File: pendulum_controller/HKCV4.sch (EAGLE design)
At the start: 56 parts, among them Q1 TPH, Q2 TPH, Q3 TPH, Q4 TPH, Q5 TPH, Q6 TPH, U1 LTC2851MPDDPBF

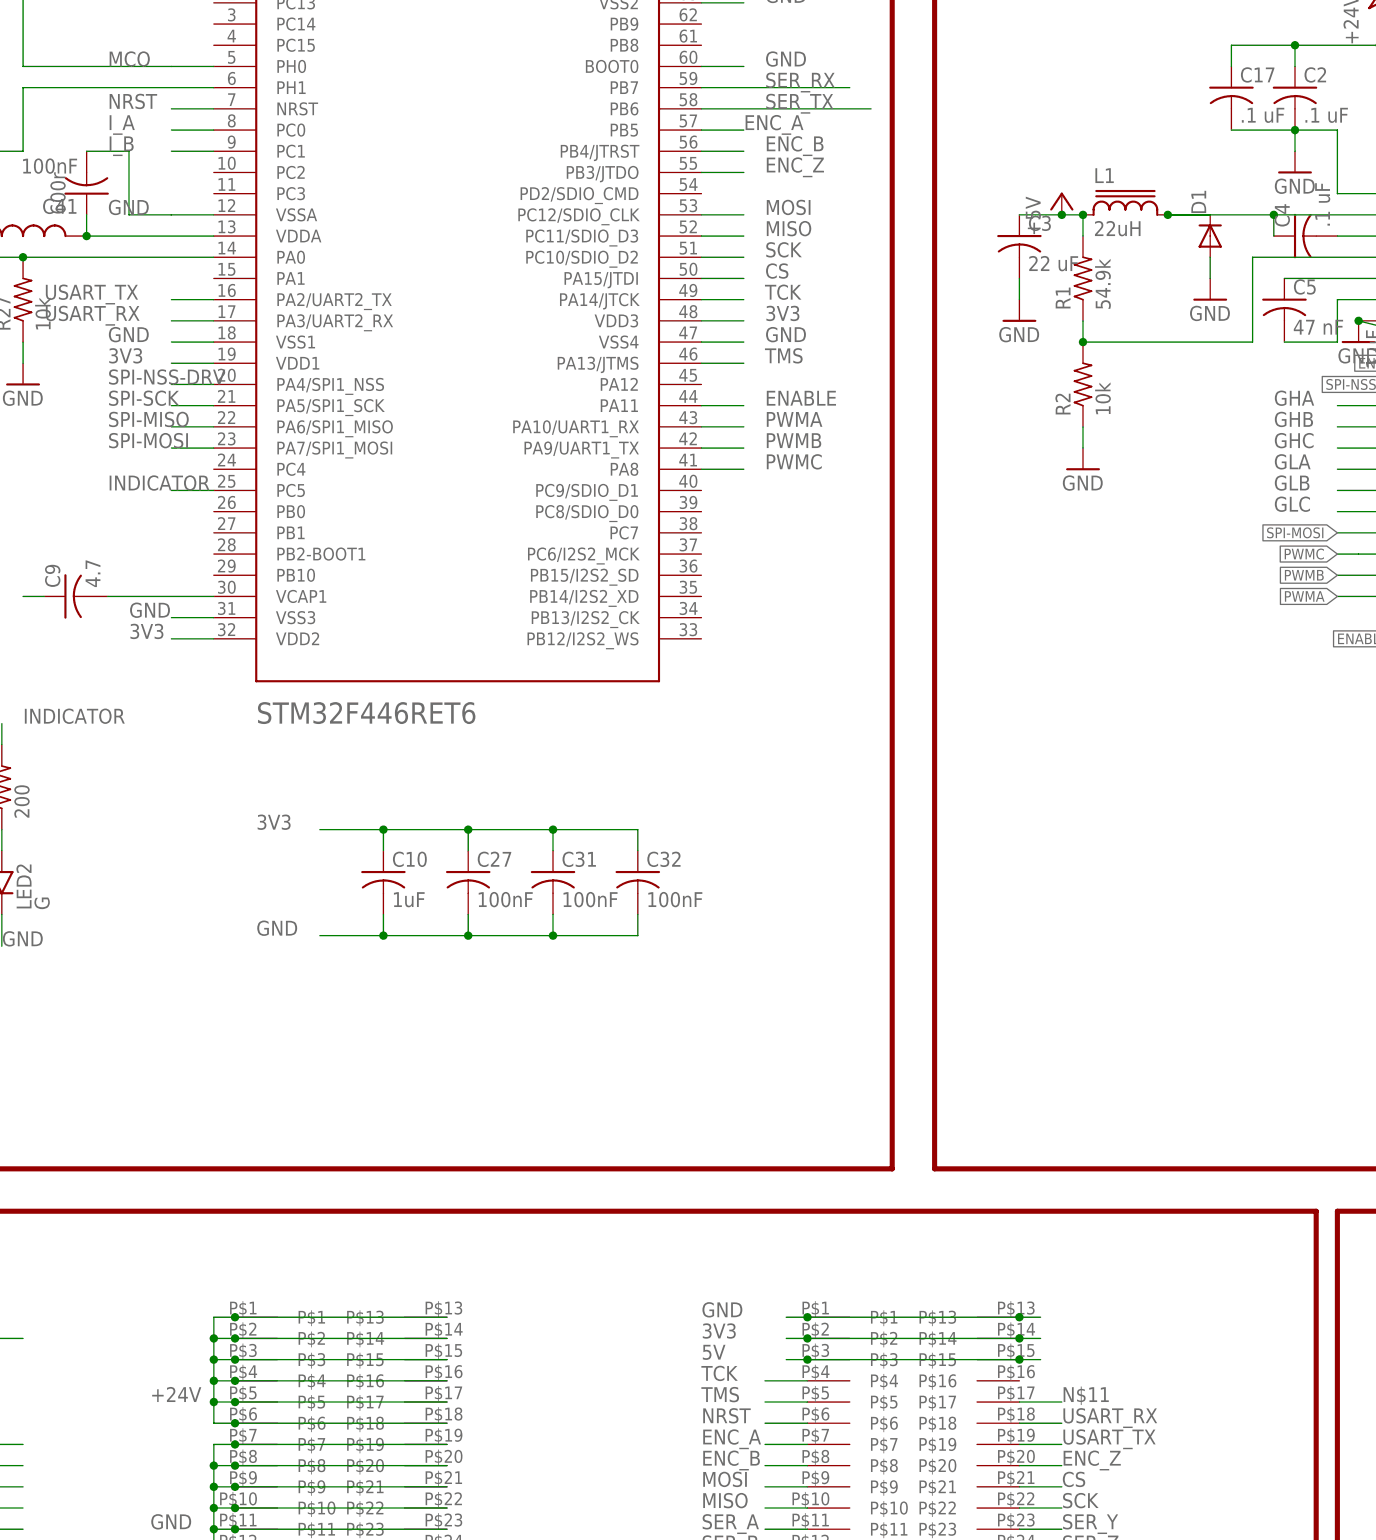
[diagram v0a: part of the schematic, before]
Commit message: updated boards
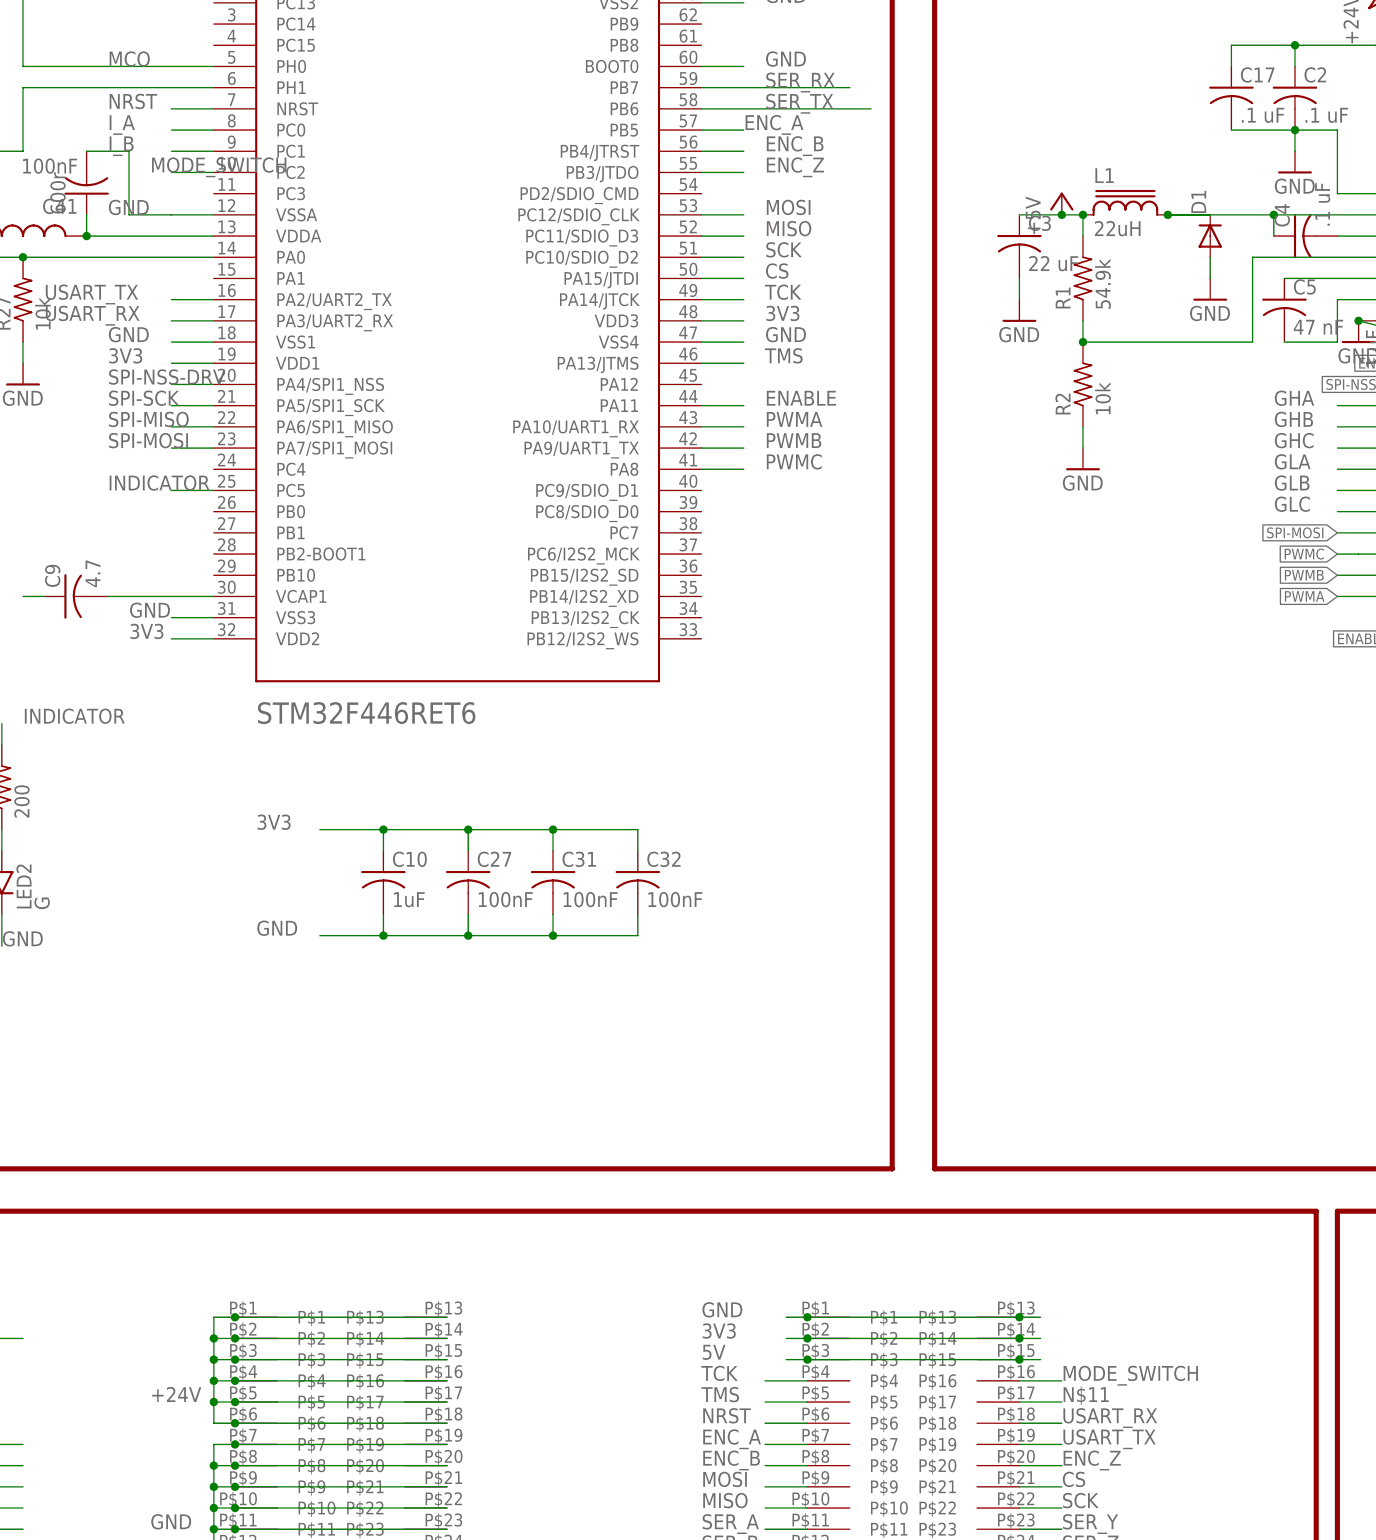
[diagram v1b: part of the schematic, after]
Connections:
- new net MODE_SWITCH: U$2.P$16, U$3.PC2
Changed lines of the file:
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@@
+</segment>
+</net>
+<net name="MODE_SWITCH" class="0">
+<segment>
+<pinref part="U$2" gate="G$1" pin="P$16"/>
+<wire x1="160.02" y1="-20.32" x2="165.1" y2="-20.32" width="0.1524" layer="91"/>
+<label x="165.1" y="-20.32" size="1.778" layer="95"/>
+</segment>
+<segment>
+<pinref part="U$3" gate="G$1" pin="PC2"/>
+<wire x1="63.5" y1="124.46" x2="58.42" y2="124.46" width="0.1524" layer="91"/>
+<label x="55.88" y="124.46" size="1.778" layer="95"/>
 </segment>
 </net>
